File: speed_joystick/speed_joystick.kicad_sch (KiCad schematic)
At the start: 12 parts, among them J2 Conn_01x04, J4 Conn_01x09, SW1 JS5208, U1 Teensy3.2, U2 SN65HVD230

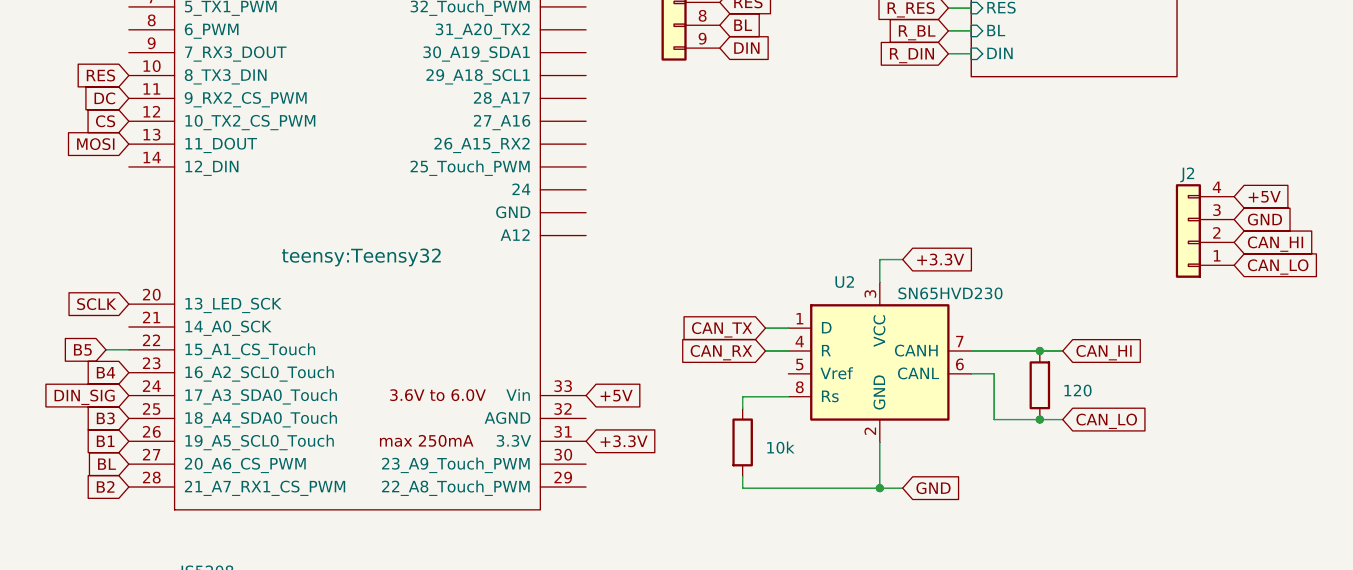
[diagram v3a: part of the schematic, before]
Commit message: created V1.2
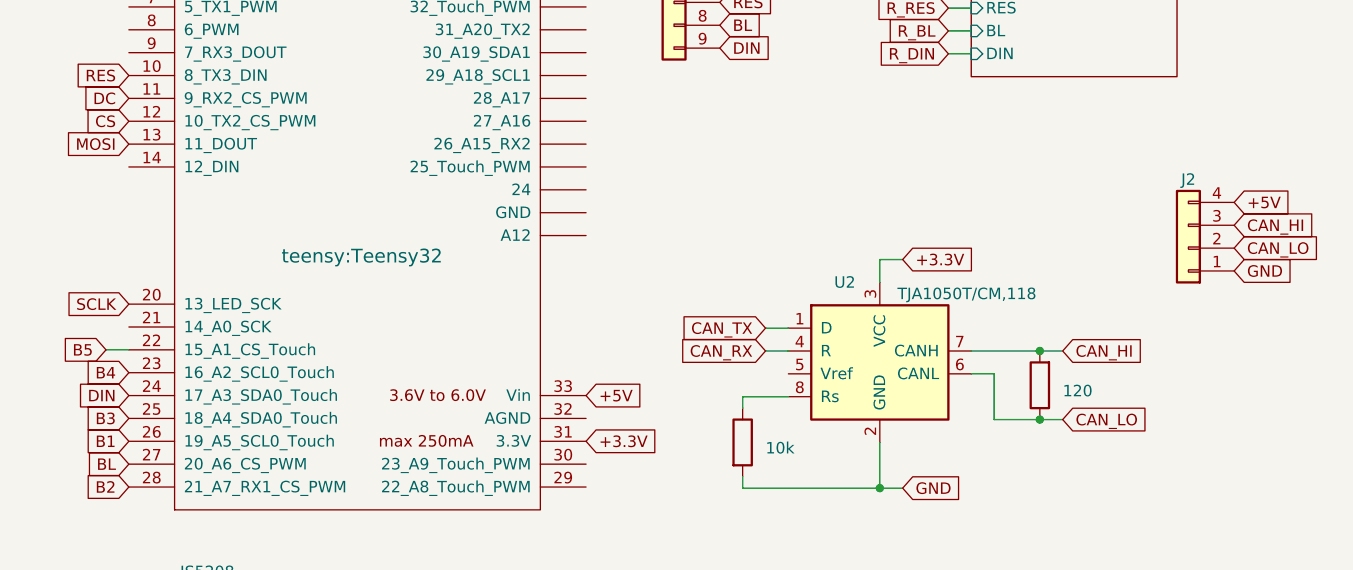
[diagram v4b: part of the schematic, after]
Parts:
- R1, R2, R3, R4, R5, R6: LCSC (none) -> C25804
- R7: LCSC (none) -> C17437
- SW1: LCSC (none) -> C3029619
- U2: value SN65HVD230 -> TJA1050T/CM,118; LCSC (none) -> C6952
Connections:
- net DIN_SIG is gone; now on net DIN: U1.24 (17_A3_SDA0_Touch)
- net CAN_HI: now also J2.3 (Pin_3); no longer J2.2 (Pin_2)
- net CAN_LO: now also J2.2 (Pin_2); no longer J2.1 (Pin_1)
- net GND: now also J2.1 (Pin_1); no longer J2.3 (Pin_3)
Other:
- moved on the sheet: J2
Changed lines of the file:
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@@
     )
   )
-  (global_label "+5V" (shape input) (at 161.29 59.055 0) (fields_autoplaced)
-    (effects (font (size 1.27 1.27)) (justify left))
-    (property "Intersheetrefs" "${INTERSHEET_REFS}" (at 167.4121 59.055 0)
+  (global_label "+5V" (shape input) (at 161.29 59.69 0) (fields_autoplaced)
+    (effects (font (size 1.27 1.27)) (justify left))
+    (property "Intersheetrefs" "${INTERSHEET_REFS}" (at 167.4121 59.69 0)
       (effects (font (size 1.27 1.27)) (justify left) hide)
     )
@@
     )
   )
-  (global_label "CAN_LO" (shape input) (at 161.29 66.675 0) (fields_autoplaced)
-    (effects (font (size 1.27 1.27)) (justify left))
-    (property "Intersheetrefs" "${INTERSHEET_REFS}" (at 170.5569 66.675 0)
+  (global_label "CAN_LO" (shape input) (at 161.29 64.77 0) (fields_autoplaced)
+    (effects (font (size 1.27 1.27)) (justify left))
+    (property "Intersheetrefs" "${INTERSHEET_REFS}" (at 170.5569 64.77 0)
       (effects (font (size 1.27 1.27)) (justify left) hide)
     )
@@
     )
   )
-  (global_label "CAN_HI" (shape input) (at 161.29 64.135 0) (fields_autoplaced)
-    (effects (font (size 1.27 1.27)) (justify left))
-    (property "Intersheetrefs" "${INTERSHEET_REFS}" (at 170.1336 64.135 0)
+  (global_label "CAN_HI" (shape input) (at 161.29 62.23 0) (fields_autoplaced)
+    (effects (font (size 1.27 1.27)) (justify left))
+    (property "Intersheetrefs" "${INTERSHEET_REFS}" (at 170.1336 62.23 0)
       (effects (font (size 1.27 1.27)) (justify left) hide)
     )
@@
     )
   )
-  (global_label "GND" (shape input) (at 161.29 61.595 0) (fields_autoplaced)
-    (effects (font (size 1.27 1.27)) (justify left))
-    (property "Intersheetrefs" "${INTERSHEET_REFS}" (at 167.4121 61.595 0)
+  (global_label "GND" (shape input) (at 161.29 67.31 0) (fields_autoplaced)
+    (effects (font (size 1.27 1.27)) (justify left))
+    (property "Intersheetrefs" "${INTERSHEET_REFS}" (at 167.4121 67.31 0)
       (effects (font (size 1.27 1.27)) (justify left) hide)
     )
@@
     )
   )
-  (global_label "DIN_SIG" (shape input) (at 38.481 81.153 180) (fields_autoplaced)
-    (effects (font (size 1.27 1.27)) (justify right))
-    (property "Intersheetrefs" "${INTERSHEET_REFS}" (at 28.9722 81.153 0)
+  (global_label "DIN" (shape input) (at 38.481 81.153 180) (fields_autoplaced)
+    (effects (font (size 1.27 1.27)) (justify right))
+    (property "Intersheetrefs" "${INTERSHEET_REFS}" (at 33.0241 81.153 0)
       (effects (font (size 1.27 1.27)) (justify right) hide)
     )
@@
       (effects (font (size 1.27 1.27)) hide)
     )
+    (property "LCSC" "C3029619" (at 43.18 110.49 0)
+      (effects (font (size 1.27 1.27)) hide)
+    )
     (pin "1")
     (pin "2")
@@
     )
     (property "Group#" "11" (at 52.07 120.65 0)
+      (effects (font (size 1.27 1.27)) hide)
+    )
+    (property "LCSC" "C25804" (at 52.07 120.65 0)
       (effects (font (size 1.27 1.27)) hide)
     )
@@
       (effects (font (size 1.27 1.27)) hide)
     )
+    (property "LCSC" "C25804" (at 106.68 86.36 0)
+      (effects (font (size 1.27 1.27)) hide)
+    )
     (pin "1")
     (pin "2")
@@
       (effects (font (size 1.27 1.27)) hide)
     )
+    (property "LCSC" "C17437" (at 139.7 80.01 0)
+      (effects (font (size 1.27 1.27)) hide)
+    )
     (pin "1")
     (pin "2")
@@
       (effects (font (size 1.27 1.27)) hide)
     )
+    (property "LCSC" "C25804" (at 52.07 125.73 0)
+      (effects (font (size 1.27 1.27)) hide)
+    )
     (pin "1")
     (pin "2")
@@
       (effects (font (size 1.27 1.27)) hide)
     )
+    (property "LCSC" "C25804" (at 52.07 128.27 0)
+      (effects (font (size 1.27 1.27)) hide)
+    )
     (pin "1")
     (pin "2")
@@
       (effects (font (size 1.27 1.27)) (justify left))
     )
-    (property "Value" "SN65HVD230" (at 123.8759 69.85 0)
+    (property "Value" "TJA1050T/CM,118" (at 123.8759 69.85 0)
       (effects (font (size 1.27 1.27)) (justify left))
     )
@@
       (effects (font (size 1.27 1.27)) hide)
     )
-    (property "Datasheet" "http://www.ti.com/lit/ds/symlink/sn65hvd230.pdf" (at 119.38 66.04 0)
+    (property "Datasheet" "https://jlcpcb.com/partdetail/NxpSemicon-TJA1050T_CM118/C6952#:~:text=Datasheet-,Download,-Source" (at 119.38 66.04 0)
+      (effects (font (size 1.27 1.27)) hide)
+    )
+    (property "LCSC" "C6952" (at 121.92 76.2 0)
       (effects (font (size 1.27 1.27)) hide)
     )
@@
     )
   )
-  (symbol (lib_id "Connector_Generic:Conn_01x04") (at 156.21 64.135 180) (unit 1)
+  (symbol (lib_id "Connector_Generic:Conn_01x04") (at 156.21 64.77 180) (unit 1)
     (in_bom yes) (on_board yes) (dnp no) (fields_autoplaced)
-    (property "Reference" "J2" (at 156.21 56.515 0)
+    (property "Reference" "J2" (at 156.21 57.15 0)
       (effects (font (size 1.27 1.27)))
     )
-    (property "Value" "Conn_01x04" (at 156.21 56.515 0)
-      (effects (font (size 1.27 1.27)) hide)
-    )
-    (property "Footprint" "4pin:my_4_tab_edge" (at 156.21 64.135 0)
-      (effects (font (size 1.27 1.27)) hide)
-    )
-    (property "Datasheet" "~" (at 156.21 64.135 0)
+    (property "Value" "Conn_01x04" (at 156.21 57.15 0)
+      (effects (font (size 1.27 1.27)) hide)
+    )
+    (property "Footprint" "4pin:my_4_tab_edge" (at 156.21 64.77 0)
+      (effects (font (size 1.27 1.27)) hide)
+    )
+    (property "Datasheet" "~" (at 156.21 64.77 0)
       (effects (font (size 1.27 1.27)) hide)
     )
@@
       (effects (font (size 1.27 1.27)) hide)
     )
+    (property "LCSC" "C25804" (at 52.07 130.81 0)
+      (effects (font (size 1.27 1.27)) hide)
+    )
     (pin "1")
     (pin "2")
@@
       (effects (font (size 1.27 1.27)) hide)
     )
+    (property "LCSC" "C25804" (at 52.07 123.19 0)
+      (effects (font (size 1.27 1.27)) hide)
+    )
